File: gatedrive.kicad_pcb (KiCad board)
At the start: 2 copper layers, 50.8 x 54.4 mm, 28 parts, among them IC1 HCPL-316J, IC2 IXDD614PI, p1 POWER SUPPLY CONNECTOR., p2 IGBT CONNECTOR., p3 CONTROLLER CONNECTOR.

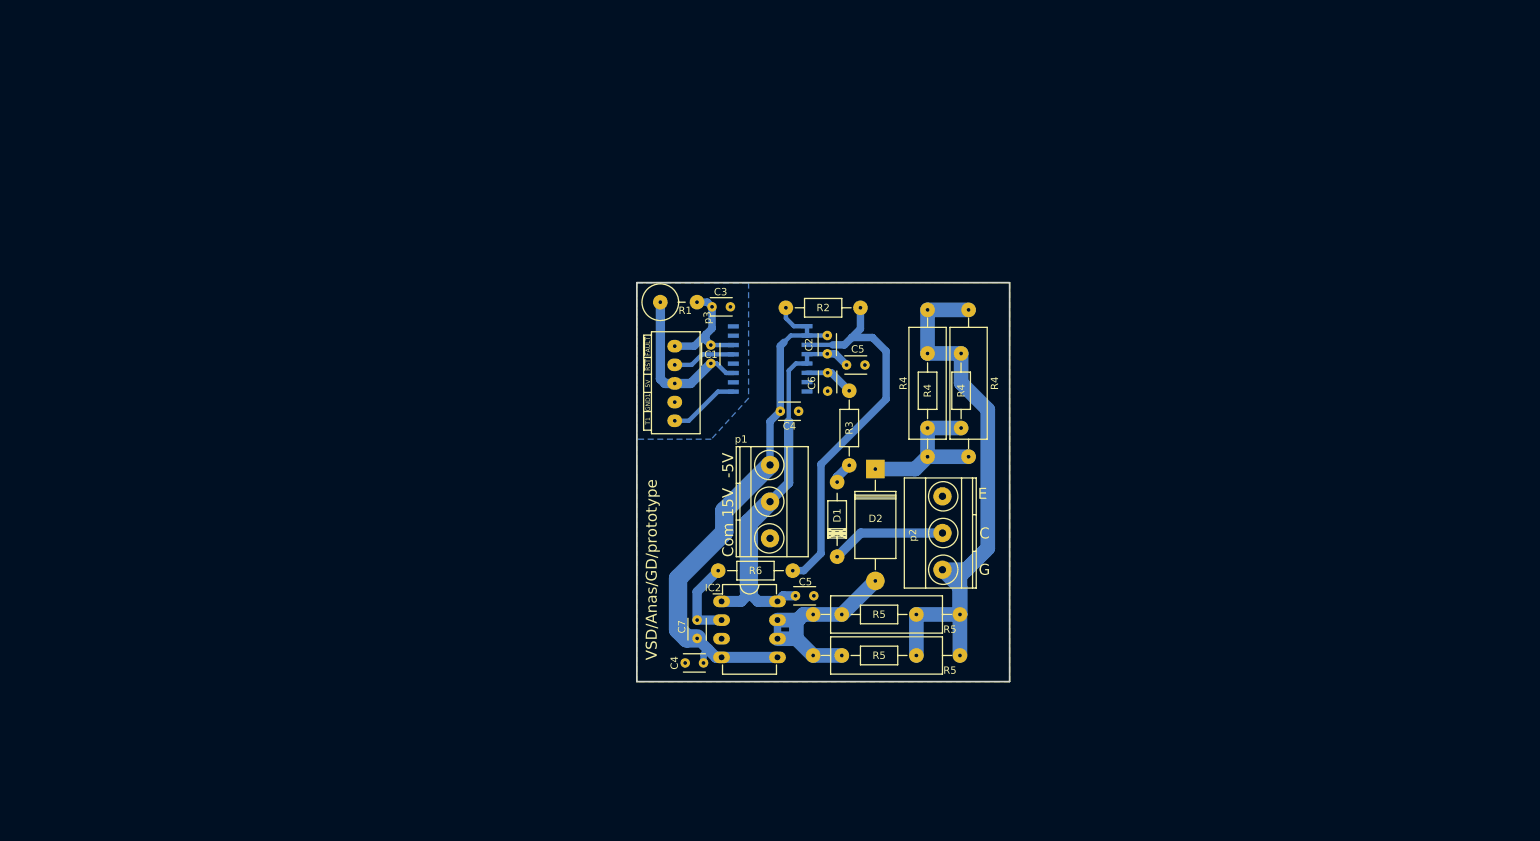
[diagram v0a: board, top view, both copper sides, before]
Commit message: cleaning the repo
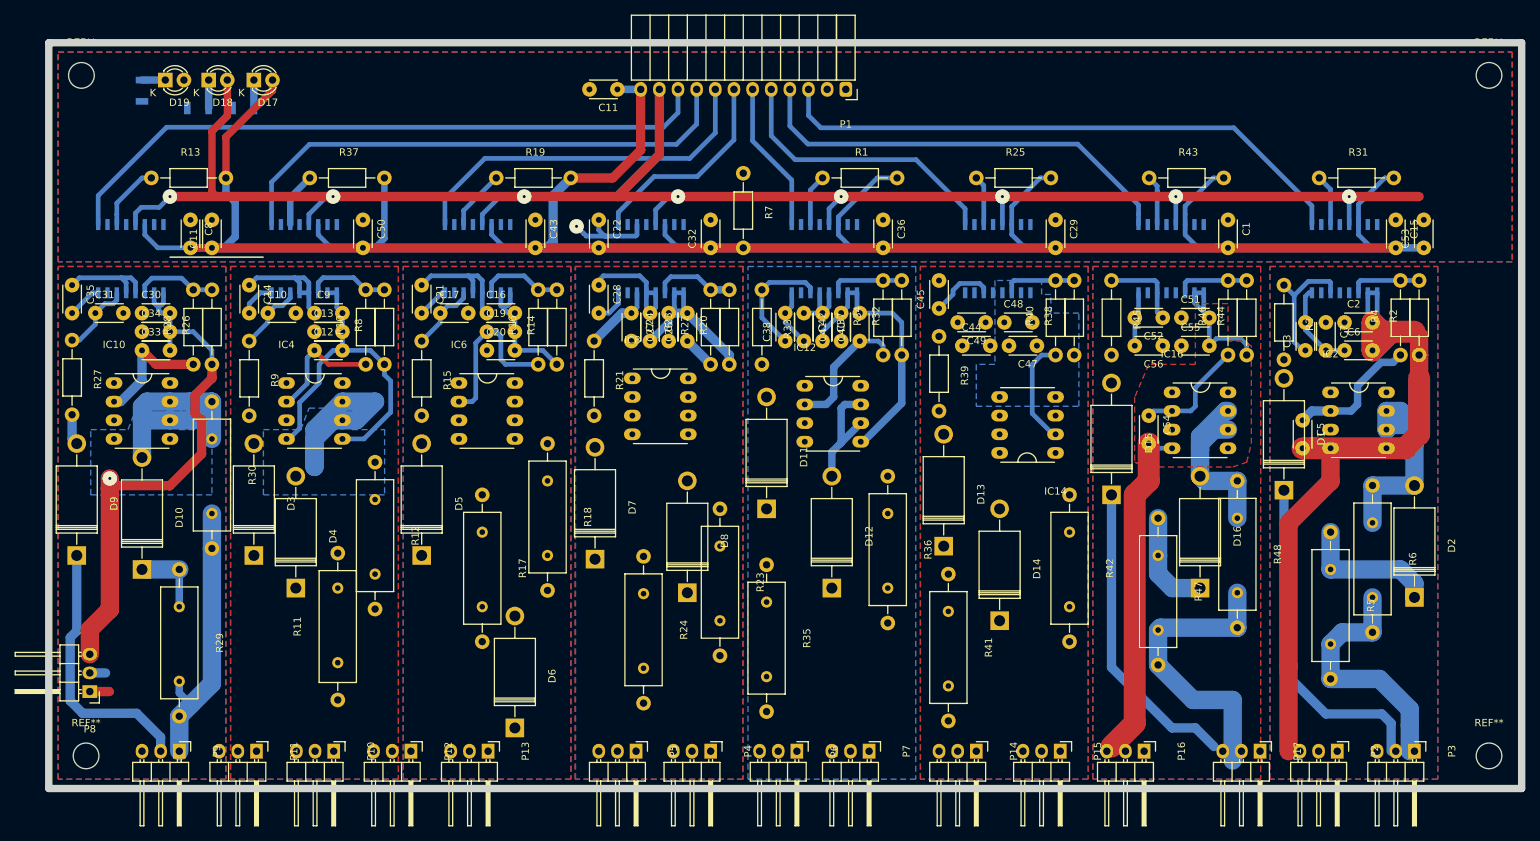
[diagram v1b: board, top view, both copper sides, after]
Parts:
- removed C4 (x2): 0.1uF, Capacitors_ThroughHole:C_Disc_D3_P2.5
- removed the C5 at (140.8, 113.5)
- removed the C5 at (147.7, 82.1)
- removed the R4 at (163.3, 85.6)
- removed the R4 at (158.8, 84.6)
- removed the R4 at (164.3, 84.6)
- removed the R4 at (158.8, 85.6)
- removed the R5 at (152.1, 116.1)
- removed the R5 at (153.2, 121.7)
- removed the R5 at (153.2, 116.1)
- removed the R5 at (152.1, 121.7)
- removed p1: POWER SUPPLY CONNECTOR., Terminal_Blocks:TerminalBlock_Pheonix_MKDS1.5-3pol
- removed p2: IGBT CONNECTOR., Terminal_Blocks:TerminalBlock_Pheonix_MKDS1.5-3pol
- removed p3: CONTROLLER CONNECTOR., Socket_Strips:Socket_Strip_Straight_1x05
- added C10: 100pF, gatedrive:C_Disc, F.Cu at (68.9, 75.0)
- added C11: 330pF, gatedrive:C_Disc, F.Cu at (61.3, 66.1)
- added C11: 330pF, gatedrive:C_Disc, F.Cu at (116.5, 44.5)
- added C12: 10nF, gatedrive:C_Disc, F.Cu at (75.2, 80.1)
- added C13: 0.1uF, gatedrive:C_Disc, F.Cu at (75.2, 77.6)
- added C14: 0.1uF, gatedrive:C_Disc, F.Cu at (66.3, 71.2)
- added C15: 0.1uF, gatedrive:C_Disc, F.Cu at (222.5, 62.3)
- added C16: 0.1uF, gatedrive:C_Disc, F.Cu at (98.7, 75.0)
- added C17: 100pF, gatedrive:C_Disc, F.Cu at (92.4, 75.0)
- added C19: 10nF, gatedrive:C_Disc, F.Cu at (98.7, 77.6)
- added C20: 0.1uF, gatedrive:C_Disc, F.Cu at (98.7, 80.1)
- added C21: 0.1uF, gatedrive:C_Disc, F.Cu at (89.8, 71.2)
- added C22: 0.1uF, gatedrive:C_Disc, F.Cu at (114.0, 62.3)
- added C23: 0.1uF, gatedrive:C_Disc, F.Cu at (120.9, 75.0)
- added C24: 100pF, gatedrive:C_Disc, F.Cu at (118.4, 75.0)
- added C26: 10nF, gatedrive:C_Disc, F.Cu at (126.0, 78.8)
- added C27: 0.1uF, gatedrive:C_Disc, F.Cu at (123.5, 78.8)
- added C28: 0.1uF, gatedrive:C_Disc, F.Cu at (114.0, 71.2)
- added C29: 0.1uF, gatedrive:C_Disc, F.Cu at (176.2, 62.3)
- added C30: 0.1uF, gatedrive:C_Disc, F.Cu at (51.7, 75.0)
- added C31: 100pF, gatedrive:C_Disc, F.Cu at (45.4, 75.0)
- added C32: 330pF, gatedrive:C_Disc, F.Cu at (129.2, 66.1)
- added C33: 10nF, gatedrive:C_Disc, F.Cu at (51.7, 80.1)
- added C34: 0.1uF, gatedrive:C_Disc, F.Cu at (51.7, 77.6)
- added C35: 0.1uF, gatedrive:C_Disc, F.Cu at (42.2, 71.2)
- added C36: 0.1uF, gatedrive:C_Disc, F.Cu at (152.7, 62.3)
- added C37: 0.1uF, gatedrive:C_Disc, F.Cu at (144.4, 75.0)
- added C38: 100pF, gatedrive:C_Disc, F.Cu at (139.4, 78.8)
- added C40: 10nF, gatedrive:C_Disc, F.Cu at (149.5, 78.8)
- added C41: 0.1uF, gatedrive:C_Disc, F.Cu at (147.0, 78.8)
- added C42: 0.1uF, gatedrive:C_Disc, F.Cu at (141.9, 75.0)
- added C43: 0.1uF, gatedrive:C_Disc, F.Cu at (105.3, 62.3)
- added C44: 0.1uF, gatedrive:C_Disc, F.Cu at (163.5, 79.5)
- added C45: 100pF, gatedrive:C_Disc, F.Cu at (160.3, 74.4)
- added C47: 10nF, gatedrive:C_Disc, F.Cu at (173.6, 79.5)
- added C48: 0.1uF, gatedrive:C_Disc, F.Cu at (169.2, 76.3)
- added C49: 0.1uF, gatedrive:C_Disc, F.Cu at (166.7, 76.3)
- added C5: 10nF, gatedrive:C_Disc, F.Cu at (209.8, 89.6)
- added C50: 0.1uF, gatedrive:C_Disc, F.Cu at (81.8, 62.3)
- added C51: 0.1uF, gatedrive:C_Disc, F.Cu at (193.3, 75.7)
- added C52: 100pF, gatedrive:C_Disc, F.Cu at (190.8, 75.7)
- added C53: 330pF, gatedrive:C_Disc, F.Cu at (226.4, 66.1)
- added C54: 10nF, gatedrive:C_Disc, F.Cu at (188.9, 89.0)
- added C55: 0.1uF, gatedrive:C_Disc, F.Cu at (193.3, 79.5)
- added C56: 0.1uF, gatedrive:C_Disc, F.Cu at (190.8, 79.5)
- added C8: 0.1uF, gatedrive:C_Disc, F.Cu at (58.3, 62.3)
- added C9: 0.1uF, gatedrive:C_Disc, F.Cu at (75.2, 75.0)
- added D10: ~, Diodes_ThroughHole:Diode_DO-201AD_Horizontal_RM15, F.Cu at (51.7, 109.9)
- added D11: RGPO2-20, Diodes_ThroughHole:Diode_DO-201AD_Horizontal_RM15, F.Cu at (136.8, 101.7)
- added D12: ~, Diodes_ThroughHole:Diode_DO-201AD_Horizontal_RM15, F.Cu at (145.7, 112.5)
- added D13: RGPO2-20, Diodes_ThroughHole:Diode_DO-201AD_Horizontal_RM15, F.Cu at (161.0, 106.8)
- added D14: ~, Diodes_ThroughHole:Diode_DO-201AD_Horizontal_RM15, F.Cu at (168.6, 116.9)
- added D15: RGPO2-20, Diodes_ThroughHole:Diode_DO-201AD_Horizontal_RM15, F.Cu at (183.8, 99.8)
- added D16: ~, Diodes_ThroughHole:Diode_DO-201AD_Horizontal_RM15, F.Cu at (195.9, 112.5)
- added D17: LED, LEDs:LED-3MM, F.Cu at (67.0, 43.3)
- added D18: LED, LEDs:LED-3MM, F.Cu at (60.8, 43.3)
- added D19: LED, LEDs:LED-3MM, F.Cu at (54.9, 43.3)
- added D3: RGPO2-20, Diodes_ThroughHole:Diode_DO-201AD_Horizontal_RM15, F.Cu at (67.0, 108.0)
- added D4: ~, Diodes_ThroughHole:Diode_DO-201AD_Horizontal_RM15, F.Cu at (72.7, 112.5)
- added D5: RGPO2-20, Diodes_ThroughHole:Diode_DO-201AD_Horizontal_RM15, F.Cu at (89.8, 108.0)
- added D6: ~, Diodes_ThroughHole:Diode_DO-201AD_Horizontal_RM15, F.Cu at (102.5, 131.5)
- added D7: RGPO2-20, Diodes_ThroughHole:Diode_DO-201AD_Horizontal_RM15, F.Cu at (113.4, 108.5)
- added D8: ~, Diodes_ThroughHole:Diode_DO-201AD_Horizontal_RM15, F.Cu at (126.0, 113.1)
- added D9: RGPO2-20, Diodes_ThroughHole:Diode_DO-201AD_Horizontal_RM15, F.Cu at (42.8, 108.0)
- added IC10: IXDD614PI, gatedrive:DIP-8_W7.62mm_LongPads, F.Cu at (47.9, 84.5)
- added IC11: HCPL-316J, Housings_SOIC:SOIC-16_7.5x10.3mm_Pitch1.27mm, B.Cu at (144.7, 67.6)
- added IC12: IXDD614PI, gatedrive:DIP-8_W7.62mm_LongPads, F.Cu at (142.0, 84.9)
- added IC13: HCPL-316J, Housings_SOIC:SOIC-16_7.5x10.3mm_Pitch1.27mm, B.Cu at (168.3, 67.6)
- added IC14: IXDD614PI, gatedrive:DIP-8_W7.62mm_LongPads, F.Cu at (176.2, 94.1)
- added IC15: HCPL-316J, Housings_SOIC:SOIC-16_7.5x10.3mm_Pitch1.27mm, B.Cu at (191.9, 67.6)
- added IC16: IXDD614PI, gatedrive:DIP-8_W7.62mm_LongPads, F.Cu at (192.1, 85.8)
- added IC3: HCPL-316J, Housings_SOIC:SOIC-16_7.5x10.3mm_Pitch1.27mm, B.Cu at (73.8, 67.6)
- added IC4: IXDD614PI, gatedrive:DIP-8_W7.62mm_LongPads, F.Cu at (71.4, 84.5)
- added IC5: HCPL-316J, Housings_SOIC:SOIC-16_7.5x10.3mm_Pitch1.27mm, B.Cu at (97.4, 67.6)
- added IC6: IXDD614PI, gatedrive:DIP-8_W7.62mm_LongPads, F.Cu at (94.9, 84.5)
- added IC7: HCPL-316J, Housings_SOIC:SOIC-16_7.5x10.3mm_Pitch1.27mm, B.Cu at (121.1, 67.6)
- added IC8: IXDD614PI, gatedrive:DIP-8_W7.62mm_LongPads, F.Cu at (118.5, 83.9)
- added IC9: HCPL-316J, Housings_SOIC:SOIC-16_7.5x10.3mm_Pitch1.27mm, B.Cu at (50.2, 67.6)
- added P1: Mic General Connector, Socket_Strips:Socket_Strip_Angled_1x12, F.Cu at (147.6, 44.5)
- added P10: CONN_01X03, Pin_Headers:Pin_Header_Angled_1x03, F.Cu at (77.8, 134.7)
- added P11: CONN_01X03, Pin_Headers:Pin_Header_Angled_1x03, F.Cu at (67.3, 134.7)
- added P12: CONN_01X03, Pin_Headers:Pin_Header_Angled_1x03, F.Cu at (88.4, 134.7)
- added P13: CONN_01X03, Pin_Headers:Pin_Header_Angled_1x03, F.Cu at (98.9, 134.7)
- added P14: CONN_01X03, Pin_Headers:Pin_Header_Angled_1x03, F.Cu at (165.4, 134.7)
- added P15: CONN_01X03, Pin_Headers:Pin_Header_Angled_1x03, F.Cu at (176.8, 134.7)
- added P16: CONN_01X03, Pin_Headers:Pin_Header_Angled_1x03, F.Cu at (188.3, 134.7)
- added P17: CONN_01X03, Pin_Headers:Pin_Header_Angled_1x03, F.Cu at (204.0, 134.7)
- added P2: CONN_01X03, Pin_Headers:Pin_Header_Angled_1x03, F.Cu at (214.6, 134.7)
- added P3: CONN_01X03, Pin_Headers:Pin_Header_Angled_1x03, F.Cu at (225.1, 134.7)
- added P4: CONN_01X03, Pin_Headers:Pin_Header_Angled_1x03, F.Cu at (129.2, 134.7)
- added P5: CONN_01X03, Pin_Headers:Pin_Header_Angled_1x03, F.Cu at (119.0, 134.7)
- added P6: CONN_01X03, Pin_Headers:Pin_Header_Angled_1x03, F.Cu at (140.9, 134.7)
- added P7: CONN_01X03, Pin_Headers:Pin_Header_Angled_1x03, F.Cu at (150.8, 134.7)
- added P8: CONN_01X03, Pin_Headers:Pin_Header_Angled_1x03, F.Cu at (44.6, 126.6)
- added P9: CONN_01X03, Pin_Headers:Pin_Header_Angled_1x03, F.Cu at (56.8, 134.7)
- added R10: 100, Resistors_ThroughHole:Resistor_Horizontal_RM10mm, F.Cu at (82.2, 82.0)
- added R11: 60, gatedrive:Resistor_multi, F.Cu at (78.4, 127.7)
- added R12: 30ohm ,0.5W, gatedrive:Resistor_multi, F.Cu at (83.5, 95.3)
- added R13: 10K, Resistors_ThroughHole:Resistor_Horizontal_RM10mm, F.Cu at (53.0, 56.6)
- added R14: 25K, Resistors_ThroughHole:Resistor_Horizontal_RM10mm, F.Cu at (108.2, 82.0)
- added R15: 100, Resistors_ThroughHole:Resistor_Horizontal_RM10mm, F.Cu at (89.8, 78.8)
- added R16: 100, Resistors_ThroughHole:Resistor_Horizontal_RM10mm, F.Cu at (105.7, 82.0)
- added R17: 60, gatedrive:Resistor_multi, F.Cu at (98.1, 99.8)
- added R18: 30ohm ,0.5W, gatedrive:Resistor_multi, F.Cu at (107.0, 92.8)
- added R19: 10K, Resistors_ThroughHole:Resistor_Horizontal_RM10mm, F.Cu at (100.0, 56.6)
- added R20: 25K, Resistors_ThroughHole:Resistor_Horizontal_RM10mm, F.Cu at (131.7, 82.0)
- added R21: 100, Resistors_ThroughHole:Resistor_Horizontal_RM10mm, F.Cu at (113.3, 78.8)
- added R22: 100, Resistors_ThroughHole:Resistor_Horizontal_RM10mm, F.Cu at (129.2, 82.0)
- added R23: 60, gatedrive:Resistor_multi, F.Cu at (130.5, 101.7)
- added R24: 30ohm ,0.5W, gatedrive:Resistor_multi, F.Cu at (120.1, 108.2)
- added R25: 10K, Resistors_ThroughHole:Resistor_Horizontal_RM10mm, F.Cu at (165.4, 56.6)
- added R26: 25K, Resistors_ThroughHole:Resistor_Horizontal_RM10mm, F.Cu at (61.3, 82.0)
- added R27: 100, Resistors_ThroughHole:Resistor_Horizontal_RM10mm, F.Cu at (42.2, 78.7)
- added R28: 100, Resistors_ThroughHole:Resistor_Horizontal_RM10mm, F.Cu at (58.7, 82.0)
- added R29: 60, gatedrive:Resistor_multi, F.Cu at (56.8, 109.9)
- added R30: 30ohm ,0.5W, gatedrive:Resistor_multi, F.Cu at (61.3, 87.1)
- added R31: 10K, Resistors_ThroughHole:Resistor_Horizontal_RM10mm, F.Cu at (212.1, 56.6)
- added R32: 25K, Resistors_ThroughHole:Resistor_Horizontal_RM10mm, F.Cu at (155.2, 80.7)
- added R33: 100, Resistors_ThroughHole:Resistor_Horizontal_RM10mm, F.Cu at (136.2, 71.8)
- added R34: 100, Resistors_ThroughHole:Resistor_Horizontal_RM10mm, F.Cu at (152.7, 80.7)
- added R35: 60, gatedrive:Resistor_multi, F.Cu at (136.8, 109.3)
- added R36: 30ohm ,0.5W, gatedrive:Resistor_multi, F.Cu at (153.3, 97.2)
- added R37: 10K, Resistors_ThroughHole:Resistor_Horizontal_RM10mm, F.Cu at (74.6, 56.6)
- added R38: 25K, Resistors_ThroughHole:Resistor_Horizontal_RM10mm, F.Cu at (178.7, 80.7)
- added R39: 100, Resistors_ThroughHole:Resistor_Horizontal_RM10mm, F.Cu at (160.3, 78.2)
- added R4: 100, Resistors_ThroughHole:Resistor_Horizontal_RM10mm, F.Cu at (223.2, 80.7)
- added R40: 100, Resistors_ThroughHole:Resistor_Horizontal_RM10mm, F.Cu at (176.2, 80.7)
- added R41: 60, gatedrive:Resistor_multi, F.Cu at (161.6, 110.6)
- added R42: 30ohm ,0.5W, gatedrive:Resistor_multi, F.Cu at (178.1, 99.8)
- added R43: 10K, Resistors_ThroughHole:Resistor_Horizontal_RM10mm, F.Cu at (188.9, 56.6)
- added R44: 25K, Resistors_ThroughHole:Resistor_Horizontal_RM10mm, F.Cu at (202.2, 80.7)
- added R45: 100, Resistors_ThroughHole:Resistor_Horizontal_RM10mm, F.Cu at (183.8, 70.6)
- added R46: 100, Resistors_ThroughHole:Resistor_Horizontal_RM10mm, F.Cu at (199.7, 80.7)
- added R47: 60, gatedrive:Resistor_multi, F.Cu at (190.2, 103.0)
- added R48: 30ohm ,0.5W, gatedrive:Resistor_multi, F.Cu at (201.0, 97.9)
- added R49: R, Resistors_SMD:R_1206, B.Cu at (65.5, 47.1)
- added R5: 60, gatedrive:Resistor_multi, F.Cu at (213.7, 104.9)
- added R50: R, Resistors_SMD:R_1206, B.Cu at (59.3, 47.1)
- added R51: R, Resistors_SMD:R_1206, B.Cu at (51.7, 44.7)
- added R7: 10K, Resistors_ThroughHole:Resistor_Horizontal_RM10mm, F.Cu at (133.6, 56.0)
- added R8: 25K, Resistors_ThroughHole:Resistor_Horizontal_RM10mm, F.Cu at (84.7, 82.0)
- added R9: 100, Resistors_ThroughHole:Resistor_Horizontal_RM10mm, F.Cu at (66.3, 78.8)
- added REF**: MountingHole_3-5mm, Mounting_Holes:MountingHole_3-5mm, F.Cu at (43.5, 42.6)
- added REF**: MountingHole_3-5mm, Mounting_Holes:MountingHole_3-5mm, F.Cu at (44.1, 135.3)
- added REF**: MountingHole_3-5mm, Mounting_Holes:MountingHole_3-5mm, F.Cu at (235.2, 135.3)
- added REF**: MountingHole_3-5mm, Mounting_Holes:MountingHole_3-5mm, F.Cu at (235.2, 42.6)
- C1, C2: footprint Capacitors_ThroughHole:C_Disc_D3_P2.5 -> gatedrive:C_Disc
- C3: value 330pF -> 100pF; footprint Capacitors_ThroughHole:C_Disc_D3_P2.5 -> gatedrive:C_Disc
- C6: value 100pF -> 0.1uF; footprint Capacitors_ThroughHole:C_Disc_D3_P2.5 -> gatedrive:C_Disc
- C7: value 10nF -> 0.1uF; footprint Capacitors_ThroughHole:C_Disc_D3_P2.5 -> gatedrive:C_Disc
- D1: footprint Diodes_ThroughHole:Diode_DO-41_SOD81_Horizontal_RM10 -> Diodes_ThroughHole:Diode_DO-201AD_Horizontal_RM15
- D2: value 1N5821 -> ~
- R1: footprint Resistors_ThroughHole:Resistor_Vertical_RM5mm -> Resistors_ThroughHole:Resistor_Horizontal_RM10mm
- R6: value 100 -> 30ohm ,0.5W; footprint Resistors_ThroughHole:Resistor_Horizontal_RM10mm -> gatedrive:Resistor_multi
- moved C7 94.8 mm to (213.0, 76.3)
- moved IC2 87.7 mm to (213.7, 85.8)
- moved R6 84.9 mm to (219.4, 98.5), turned to 270 degrees
- moved R2 81.4 mm to (225.7, 80.7), turned to 90 degrees
- moved C3 81.1 mm to (210.2, 80.1), turned to 90 degrees
- moved IC1 79.1 mm to (215.6, 67.6), turned to 270 degrees
- moved D2 75.5 mm to (225.1, 113.8), turned to 90 degrees
- moved C1 73.1 mm to (199.7, 62.3), turned to 270 degrees
- moved C2 70.6 mm to (215.6, 76.3), turned to 0 degrees
- moved C6 70.5 mm to (215.6, 80.1), turned to 0 degrees
- moved R3 62.3 mm to (207.3, 71.2)
- moved D1 61.5 mm to (207.3, 99.2)
- moved R1 25.9 mm to (144.4, 56.6)
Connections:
- C2 pad 1: 15V -> 15v1
- C2 pad 2: -5V -> -5V1
- C3 pad 1: ~FAULT -> Net-(C3-Pad1)
- C3 pad 2: GND1 -> COM1
- C6 pad 1: Net-(C6-Pad1) -> COM1
- C6 pad 2: COM -> -5V1
- C7 pad 1: Net-(C7-Pad1) -> 15v1
- C7 pad 2: -5V -> COM1
- D1 pad 1: C -> C1
- IC1 pad 10: -5V -> -5V1
- IC1 pad 12: 15V -> 15v1
- IC1 pad 13: 15V -> 15v1
- IC1 pad 14: Net-(C6-Pad1) -> Net-(C3-Pad1)
- IC1 pad 15: (no net) -> Net-(IC1-Pad15)
- IC1 pad 16: COM -> COM1
- IC1 pad 7: (no net) -> Net-(IC1-Pad7)
- IC1 pad 9: -5V -> -5V1
- IC2 pad 1: 15V -> 15v1
- IC2 pad 2: Net-(C7-Pad1) -> Net-(C5-Pad1)
- IC2 pad 3: (no net) -> 15v1
- IC2 pad 4: -5V -> -5V1
- IC2 pad 5: -5V -> -5V1
- IC2 pad 8: 15V -> 15v1
- R2 pad 1: -5V -> -5V1
- R3 pad 1: Net-(C6-Pad1) -> Net-(C3-Pad1)
- R6 pad 1: Net-(C7-Pad1) -> Net-(D2-Pad2)
- R6 pad 2: Net-(IC1-Pad11) -> G1
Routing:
- net ~FAULT: track 16.1 -> 349.6 mm
- net ~RST: track 8.57 -> 246.9 mm, vias 0 -> 8
- net -5V1: track 0.00 -> 109.5 mm
- net /T8: track 0.00 -> 90.8 mm
- net G: track 85.9 -> 0.00 mm
- net -5V: track 74.6 -> 0.00 mm
- net -5v8: track 0.00 -> 73.8 mm, vias 0 -> 1
- net /T7: track 0.00 -> 71.7 mm
- net T1: track 9.63 -> 79.8 mm
- net -5V2: track 0.00 -> 67.1 mm
- net /T2: track 0.00 -> 59.6 mm
- net 15V: track 54.3 -> 0.00 mm
- net /T6: track 0.00 -> 50.0 mm
- net -5V7: track 0.00 -> 47.1 mm
- net C1: track 0.00 -> 46.1 mm
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- added copper zone on F.Cu, net -5V2
- added copper zone on B.Cu, net -5V3
- added copper zone on B.Cu, net -5V7
- added copper zone on B.Cu, net -5v8
- added copper zone on B.Cu, net 15V2
- added copper zone on B.Cu, net 15V3
- added copper zone on B.Cu, net 15V4
- added copper zone on B.Cu, net 15V5
- added copper zone on B.Cu, net 15V6
- added copper zone on B.Cu, net 15V7
- added copper zone on B.Cu, net 15V8
- added copper zone on B.Cu, net 15v1
- added copper zone on F.Cu, net COM1
- added copper zone on F.Cu, net COM2
- added copper zone on F.Cu, net COM3
- added copper zone on F.Cu, net COM5
- added copper zone on F.Cu, net COM6
- added copper zone on F.Cu, net COM7
- added copper zone on F.Cu, net COM8
- added copper zone on F.Cu, net MICSUPP
- removed copper zone on B.Cu, net COM
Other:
- board size 50.8 x 54.4 mm -> 200.7 x 101.6 mm
- net class Default: via_dia 0.6 -> 2
- net class Gate signal added: clearance 0.2, trace_width 2, via_dia 2, via_drill 0.4
- board text removed: "-5V"
- board text removed: "14A IGBT GATE DRIVER BASED ON IXDD614PI AND HCPL-316J"
- board text removed: "15V"
- board text removed: "C"
- board text removed: "Com"
- board text removed: "E"
- board text removed: "G"
- board text removed: "VSD/Anas/GD/prototype"
- board text removed: "note that gate resistors are easily scalabe to different IGBT sizes."
